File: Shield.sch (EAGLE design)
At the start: 82 parts

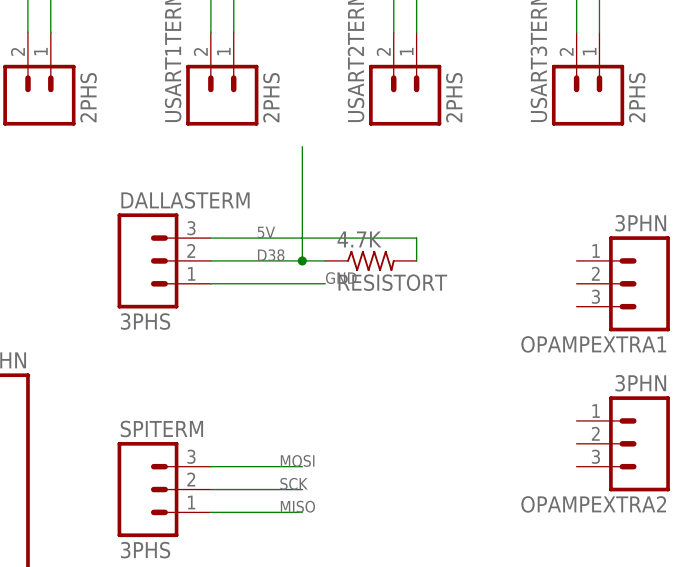
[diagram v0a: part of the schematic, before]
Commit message: Ready for Quantity Manufacturing
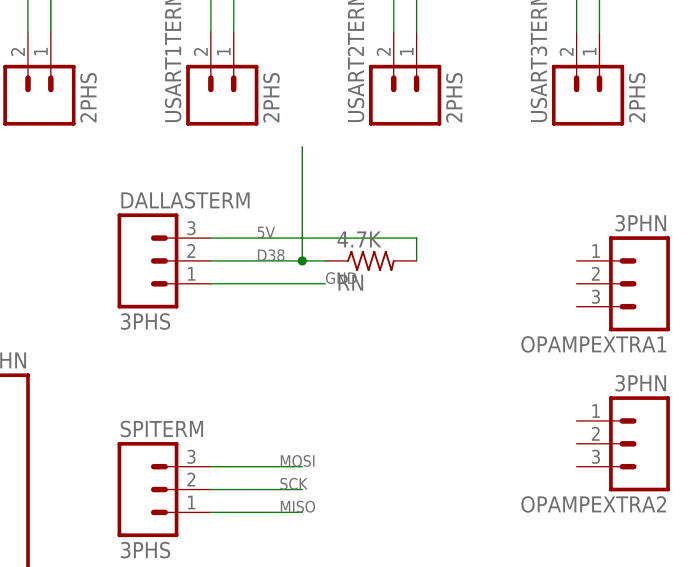
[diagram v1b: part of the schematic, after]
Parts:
- 4.7K: value RESISTORT -> RN; device LEMS:RESISTORT -> LEMS:RN
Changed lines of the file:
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@@
 <part name="OPA2TERM" library="LEMS" deviceset="3PH" device="N"/>
 <part name="DALLASTERM" library="LEMS" deviceset="3PH" device="S"/>
-<part name="4.7K" library="LEMS" deviceset="RESISTOR" device="T"/>
+<part name="4.7K" library="LEMS" deviceset="R" device="N"/>
 <part name="GND17" library="LEMS" deviceset="GND" device=""/>
 <part name="4.5VTERM" library="LEMS" deviceset="2PH" device="S"/>
